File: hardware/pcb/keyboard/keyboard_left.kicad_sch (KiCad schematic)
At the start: 27 parts, among them J1 SM04B-SRSS-TB, J2 PJ320D, J3 HRO_TYPE-C-31-M-12, J4 FH34SRJ-10S-0.5SH, SW29 PTS845, U3 DT1446-04S, U4 XC6220B331MR-G, U5 STM32G0B1KETx, Y1 NX3215SA

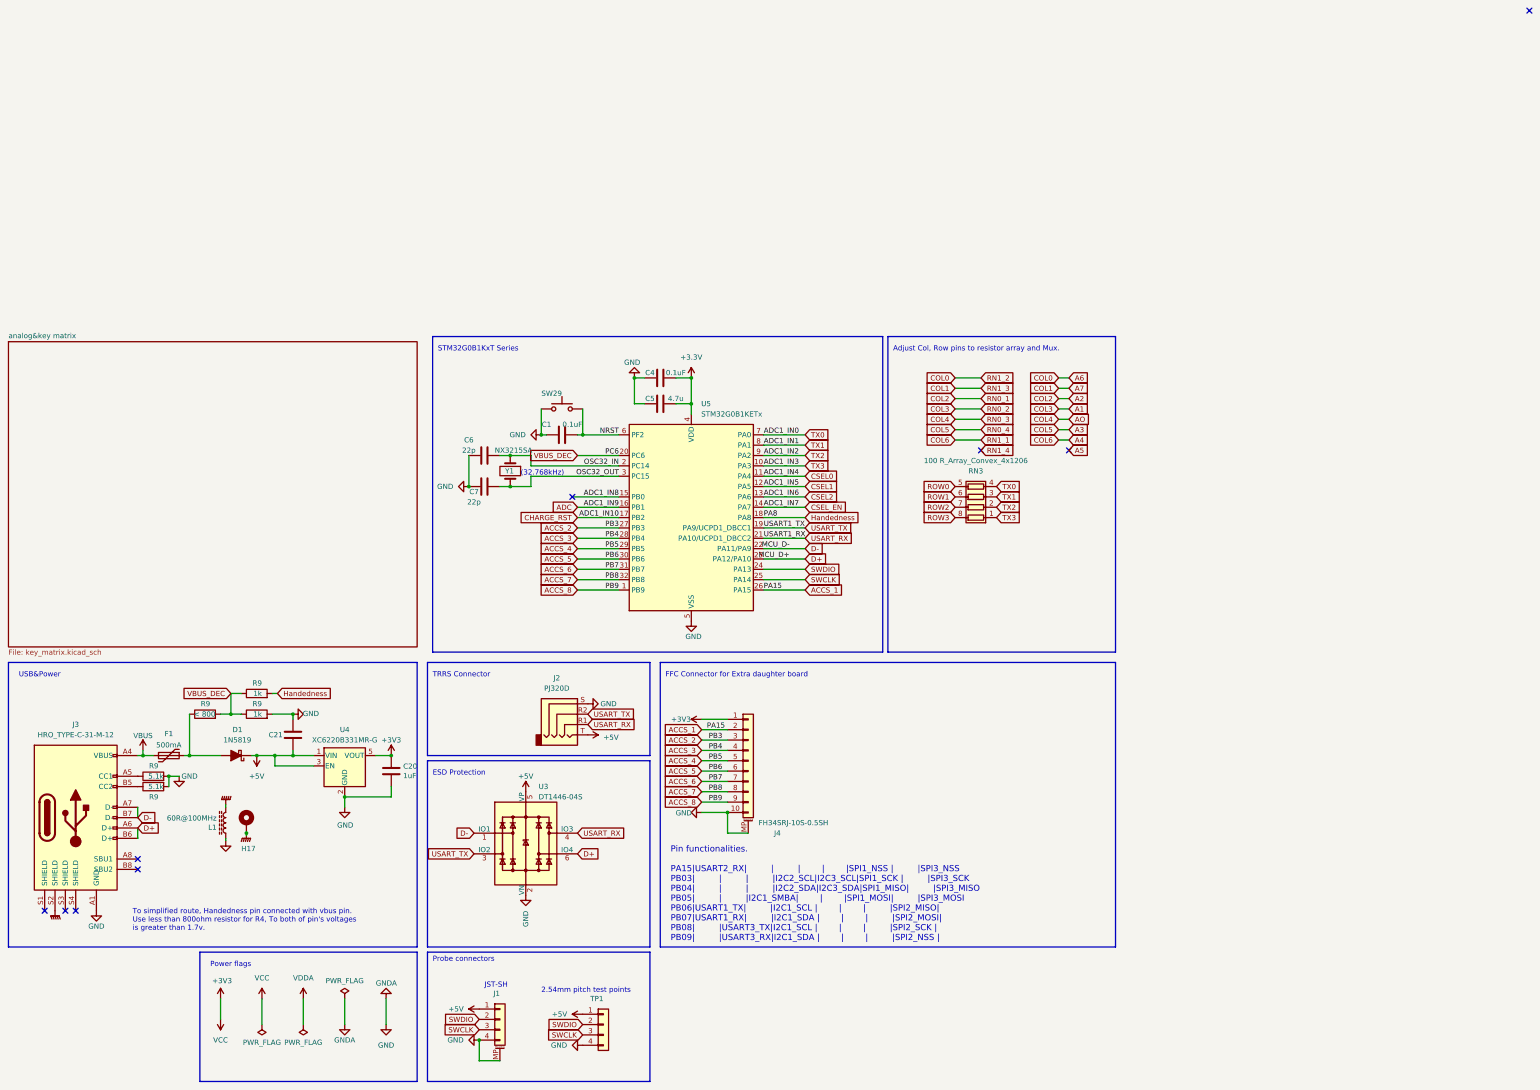
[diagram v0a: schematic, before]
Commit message: temp
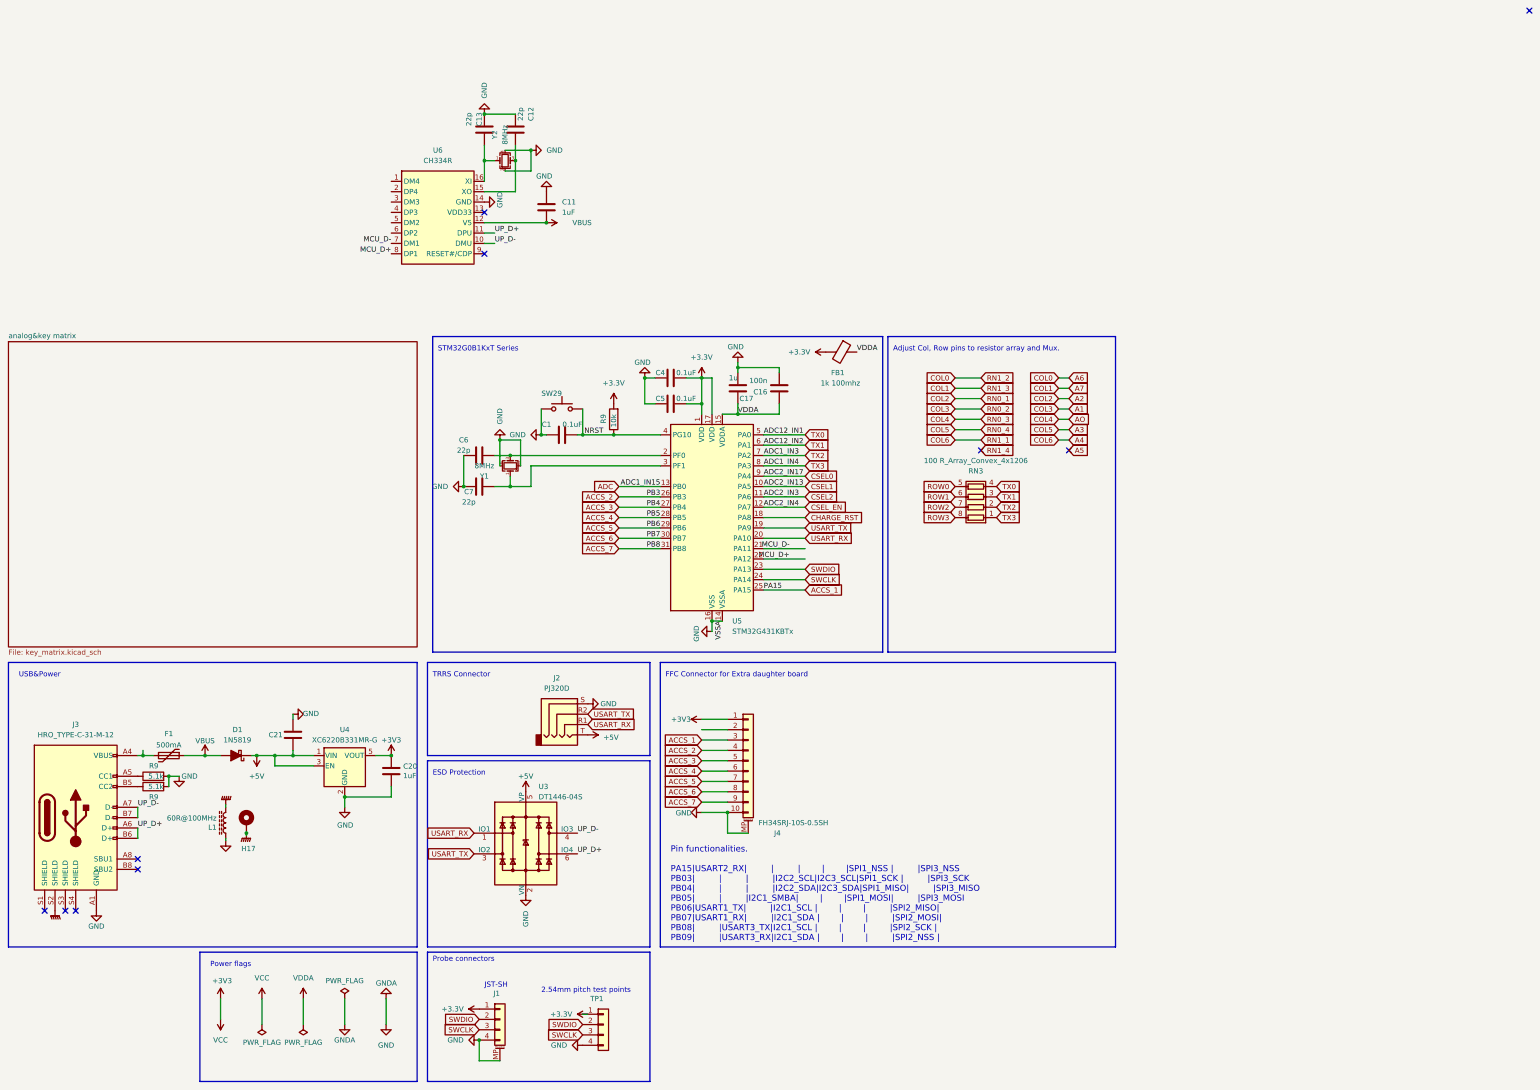
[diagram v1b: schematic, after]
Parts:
- removed R9 (x2): 1k, PCM_Resistor_SMD_AKL:R_0603_1608Metric_Pad0.98x0.95mm, symbol Device:R
- removed R9: < 800, PCM_Resistor_SMD_AKL:R_0603_1608Metric_Pad0.98x0.95mm, symbol Device:R
- removed U5: STM32G0B1KETx, PCM_Package_QFP_AKL:LQFP-32_7x7mm_P0.8mm, symbol MCU_ST_STM32G0:STM32G0B1KETx
- removed Y1: NX3215SA, PCM_Crystal_AKL:Crystal_SMD_3215-2Pin_3.2x1.5mm, symbol Device:Crystal
- added C11: 1uF, PCM_Capacitor_SMD_AKL:C_0603_1608Metric, symbol Device:C
- added C12, C13: 22p, PCM_Capacitor_SMD_AKL:C_0603_1608Metric, symbol Device:C
- added C16: 100n, PCM_Capacitor_SMD_AKL:C_0603_1608Metric, symbol Device:C
- added C17: 1u, PCM_Capacitor_SMD_AKL:C_0603_1608Metric, symbol Device:C
- added FB1: 1k 100mhz, Inductor_SMD:L_0603_1608Metric, symbol Device:FerriteBead
- added R9: 10k, PCM_Resistor_SMD_AKL:R_0603_1608Metric, symbol Device:R
- added U5: STM32G431KBTx, Package_QFP:LQFP-32_7x7mm_P0.8mm, symbol MCU_ST_STM32G4:STM32G431KBTx
- added U6: CH334R, Package_SO:QSOP-16_3.9x4.9mm_P0.635mm, symbol wch_mcu_peripheral:CH334R
- added Y1, Y2: 8MHz, PCM_Crystal_Handsoldering_AKL:Crystal_SMD_2520-4Pin_2.5x2.0mm, symbol Device:Crystal_GND24_Small
- C1, C20, C21, C4, C6, C7: footprint PCM_Capacitor_SMD_AKL:C_0603_1608Metric_Pad1.05x0.95mm -> PCM_Capacitor_SMD_AKL:C_0603_1608Metric
- C5: value 4.7u -> 0.1uF; footprint PCM_Capacitor_SMD_AKL:C_0603_1608Metric_Pad1.05x0.95mm -> PCM_Capacitor_SMD_AKL:C_0603_1608Metric
- R9: footprint PCM_Resistor_SMD_AKL:R_0603_1608Metric_Pad0.98x0.95mm -> PCM_Resistor_SMD_AKL:R_0603_1608Metric
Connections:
- net ACCS_8 is gone; now on net ACCS_7: J4.9 (Pin_9)
- net +3V3: now also J1.1 (Pin_1), TP1.1 (Pin_1), FB1.2, R9.2, U5.1 (VDD), U5.17 (VDD)
- net +5V: no longer J1.1 (Pin_1), TP1.1 (Pin_1)
- net ACCS_1: now also J4.3 (Pin_3), U5.25 (PA15); no longer J4.2 (Pin_2)
- net ACCS_2: now also J4.4 (Pin_4), U5.26 (PB3); no longer J4.3 (Pin_3)
- net ACCS_3: now also J4.5 (Pin_5), U5.27 (PB4); no longer J4.4 (Pin_4)
- net ACCS_4: now also J4.6 (Pin_6), U5.28 (PB5); no longer J4.5 (Pin_5)
- net ACCS_5: now also J4.7 (Pin_7), U5.29 (PB6); no longer J4.6 (Pin_6)
- net ACCS_6: now also J4.8 (Pin_8), U5.30 (PB7); no longer J4.7 (Pin_7)
- net ACCS_7: now also U5.31 (PB8); no longer J4.8 (Pin_8)
- net ADC: now also U5.13 (PB0)
- net CHARGE_RST: now also U5.18 (PA8)
- net CSEL0: now also U5.9 (PA4)
- net CSEL1: now also U5.10 (PA5)
- net CSEL2: now also U5.11 (PA6)
- net CSEL_EN: now also U5.12 (PA7)
- net GND: now also C11.2, C12.1, C13.1, C16.2, C17.2, U5.14 (VSSA), U5.16 (VSS), U5.32 (VSS), U6.14 (GND), Y1.2, Y1.4, Y2.2, Y2.4
- net NRST: now also R9.1, U5.4 (PG10)
- net SWCLK: now also U5.24 (PA14)
- net SWDIO: now also U5.23 (PA13)
- net TX0: now also U5.5 (PA0)
- net TX1: now also U5.6 (PA1)
- net TX2: now also U5.7 (PA2)
- net TX3: now also U5.8 (PA3)
- net USART_RX: now also U3.1 (IO1), U5.20 (PA10); no longer U3.4 (IO3)
- net USART_TX: now also U5.19 (PA9)
- net VBUS: now also D1.2 (A), F1.1, C11.1, U6.12 (V5); no longer F1.2, J3.A4 (VBUS), J3.A9 (VBUS), J3.B4 (VBUS), J3.B9 (VBUS)
- net VDDA: now also C16.1, C17.1, FB1.1, U5.15 (VDDA)
- net D+ renamed UP_D+
- net UP_D+: now also U6.11 (DPU)
- net D- renamed UP_D-
- net UP_D-: now also U3.4 (IO3), U6.10 (DMU); no longer U3.1 (IO1)
- net OSC32_IN: no longer names the net of C6.2
- net OSC32_IN: now also U5.2 (PF0), Y1.3
- net OSC32_OUT: no longer names the net of C7.2
- net OSC32_OUT: now also U5.3 (PF1), Y1.1
- new net: C12.2, U6.15 (XO), Y2.3
- new net: C13.2, U6.16 (XI), Y2.1
- new net: F1.2, J3.A4 (VBUS), J3.A9 (VBUS), J3.B4 (VBUS), J3.B9 (VBUS)
- new net MCU_D+: U5.22 (PA12), U6.8 (DP1)
- new net MCU_D-: U5.21 (PA11), U6.7 (DM1)
- no-connect marks 9 -> 10
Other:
- note removed: "(32.768kHz)"
- note removed: "To simplified route, Handedness pin connected with vbus pin. Use less than 800ohm resistor for R4, To both of pin's voltages is greater than 1.7v."
- moved on the sheet: C4, C5, C6, C7

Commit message: Left init
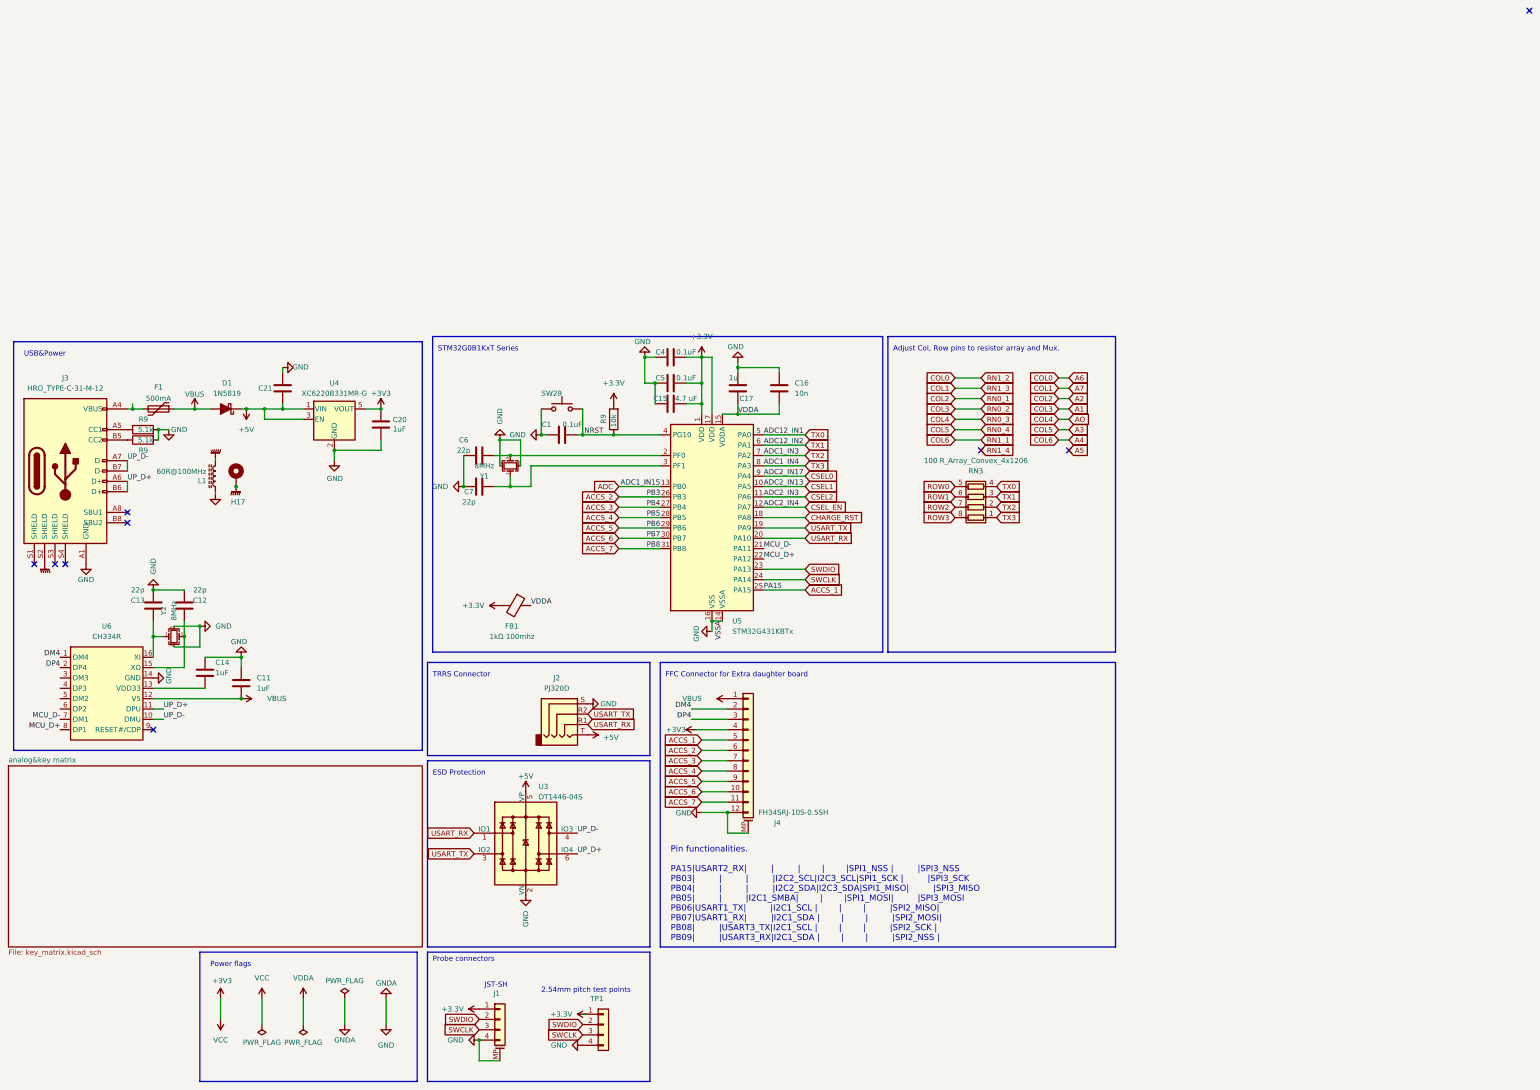
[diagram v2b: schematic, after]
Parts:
- removed J4: FH34SRJ-10S-0.5SH, ec_parts:HRS_FH34SRJ-10S-0.5SH(50), symbol Connector_Generic_MountingPin:Conn_01x10_MountingPin
- added C14: 1uF, PCM_Capacitor_SMD_AKL:C_0603_1608Metric, symbol Device:C
- added C15: 4.7 uF, PCM_Capacitor_SMD_AKL:C_0603_1608Metric, symbol Device:C
- added J4: FH34SRJ-10S-0.5SH, ec_parts:HRS_FH34SRJ-12S-0.5SH(50), symbol Connector_Generic_MountingPin:Conn_01x12_MountingPin
- C16: value 100n -> 10n
- FB1: value 1k 100mhz -> 1kΩ 100mhz
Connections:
- net +3V3: now also C15.1, J4.4 (Pin_4)
- net ACCS_1: now also J4.5 (Pin_5)
- net ACCS_2: now also J4.6 (Pin_6)
- net ACCS_3: now also J4.7 (Pin_7)
- net ACCS_4: now also J4.8 (Pin_8)
- net ACCS_5: now also J4.9 (Pin_9)
- net ACCS_6: now also J4.10 (Pin_10)
- net ACCS_7: now also J4.11 (Pin_11)
- net GND: now also C14.2, C15.2, J4.12 (Pin_12), J4.MP (MountPin)
- net VBUS: now also J4.1 (Pin_1)
- net DM4: now reaches U6.1 (DM4)
- net DM4: now also J4.2 (Pin_2)
- net at U6.13 (VDD33): now also C14.1
- net DP4: now reaches U6.2 (DP4)
- net DP4: now also J4.3 (Pin_3)
- no-connect marks 10 -> 9
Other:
- moved on the sheet: C11, C12, C13, C20, C21, C4, C5, D1, F1, FB1, H17, J3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

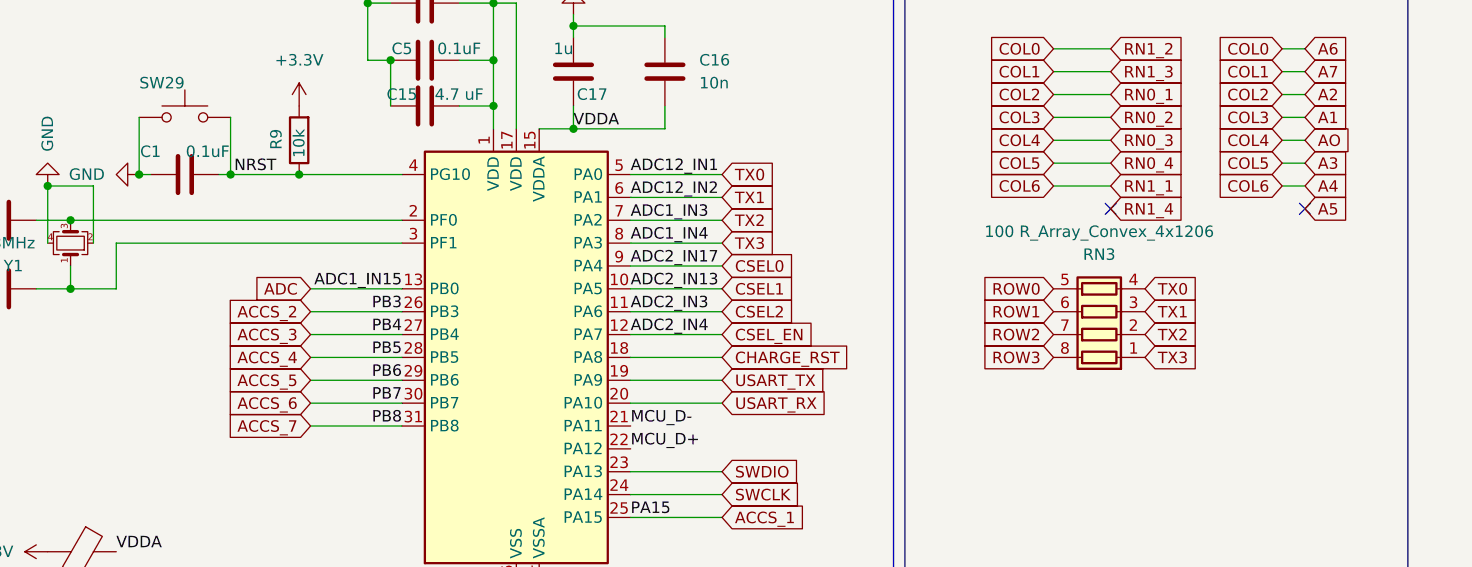
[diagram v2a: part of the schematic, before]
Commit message: Right init
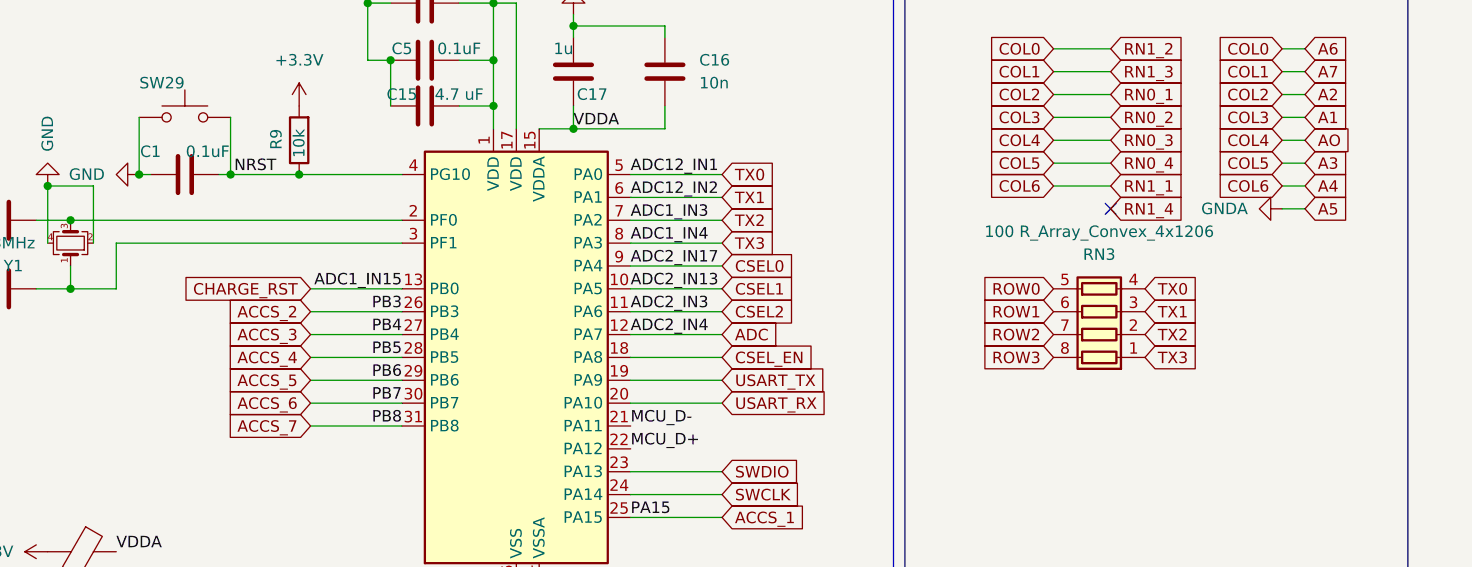
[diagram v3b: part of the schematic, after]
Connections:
- net ADC: now also U5.12 (PA7); no longer U5.13 (PB0)
- net CHARGE_RST: now also U5.13 (PB0); no longer U5.18 (PA8)
- net CSEL_EN: now also U5.18 (PA8); no longer U5.12 (PA7)
- no-connect marks 9 -> 8
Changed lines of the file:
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@@
   (junction (at 69.85 92.71) (diameter 0) (color 0 0 0 0)
   )
-  (no_connect (at 273.05 41.91))
   (no_connect (at 41.91 59.69))
   (no_connect (at 251.46 41.91))
@@
     (stroke (width 0) (type default))
   )
+  (wire (pts (xy 270.51 41.91) (xy 273.05 41.91))
+    (stroke (width 0) (type default))
+  )
   (wire (pts (xy 171.45 25.4) (xy 168.91 25.4))
     (stroke (width 0) (type default))
@@
     (effects (font (size 1.27 1.27)) (justify right bottom))
   )
+  (global_label "ADC" (shape input) (at 208.28 55.88 0) (fields_autoplaced)
+    (effects (font (size 1.27 1.27)) (justify left))
+    (property "Intersheetrefs" "${INTERSHEET_REFS}" (at 213.5971 55.88 0)
+      (effects (font (size 1.27 1.27)) (justify left) hide)
+    )
+  )
   (global_label "SWDIO" (shape input) (at 208.28 71.12 0) (fields_autoplaced)
     (effects (font (size 1.27 1.27)) (justify left))
@@
     )
   )
-  (global_label "CSEL_EN" (shape input) (at 208.28 55.88 0) (fields_autoplaced)
-    (effects (font (size 1.27 1.27)) (justify left))
-    (property "Intersheetrefs" "${INTERSHEET_REFS}" (at 217.8753 55.88 0)
+  (global_label "CSEL_EN" (shape input) (at 208.28 58.42 0) (fields_autoplaced)
+    (effects (font (size 1.27 1.27)) (justify left))
+    (property "Intersheetrefs" "${INTERSHEET_REFS}" (at 217.8753 58.42 0)
       (effects (font (size 1.27 1.27)) (justify left) hide)
     )
@@
     )
   )
-  (global_label "ADC" (shape input) (at 162.56 50.8 180) (fields_autoplaced)
-    (effects (font (size 1.27 1.27)) (justify right))
-    (property "Intersheetrefs" "${INTERSHEET_REFS}" (at 157.2429 50.8 0)
-      (effects (font (size 1.27 1.27)) (justify right) hide)
-    )
-  )
   (global_label "ACCS_3" (shape input) (at 182.88 118.11 180) (fields_autoplaced)
     (effects (font (size 1.27 1.27)) (justify right))
@@
     )
   )
+  (global_label "CHARGE_RST" (shape input) (at 162.56 50.8 180) (fields_autoplaced)
+    (effects (font (size 1.27 1.27)) (justify right))
+    (property "Intersheetrefs" "${INTERSHEET_REFS}" (at 149.7562 50.8 0)
+      (effects (font (size 1.27 1.27)) (justify right) hide)
+    )
+  )
   (global_label "TX2" (shape input) (at 255.27 55.88 0) (fields_autoplaced)
     (effects (font (size 1.27 1.27)) (justify left))
@@
     (property "Intersheetrefs" "${INTERSHEET_REFS}" (at 223.52 166.37 0)
       (effects (font (size 1.27 1.27)) hide)
-    )
-  )
-  (global_label "CHARGE_RST" (shape input) (at 208.28 58.42 0) (fields_autoplaced)
-    (effects (font (size 1.27 1.27)) (justify left))
-    (property "Intersheetrefs" "${INTERSHEET_REFS}" (at 221.0838 58.42 0)
-      (effects (font (size 1.27 1.27)) (justify left) hide)
     )
   )
@@
         )
       )
+    )
+  )
+  (symbol (lib_id "power:GNDA") (at 270.51 41.91 270) (unit 1)
+    (in_bom yes) (on_board yes) (dnp no)
+    (property "Reference" "#PWR052" (at 264.16 41.91 0)
+      (effects (font (size 1.27 1.27)) hide)
+    )
+    (property "Value" "GNDA" (at 266.7 41.91 90)
+      (effects (font (size 1.27 1.27)) (justify right))
+    )
+    (property "Footprint" "" (at 270.51 41.91 0)
+      (effects (font (size 1.27 1.27)) hide)
+    )
+    (property "Datasheet" "" (at 270.51 41.91 0)
+      (effects (font (size 1.27 1.27)) hide)
+    )
+    (pin "1")
+    (instances
+      (project "keyboard_left"
+        (path "/852dabbf-de45-4470-8176-59d37a754407"
+          (reference "#PWR052") (unit 1)
+        )
+        (path "/852dabbf-de45-4470-8176-59d37a754407/ac97752b-a16f-44ee-ad7e-0bcdbcea7979"
+          (reference "#PWR043") (unit 1)
+        )
+      )
